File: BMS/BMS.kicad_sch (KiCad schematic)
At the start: 112 parts, among them IC1 L9963E-TR, T1 Transformer_1P_1S, T2 Transformer_1P_1S, U1 QRE1113GR

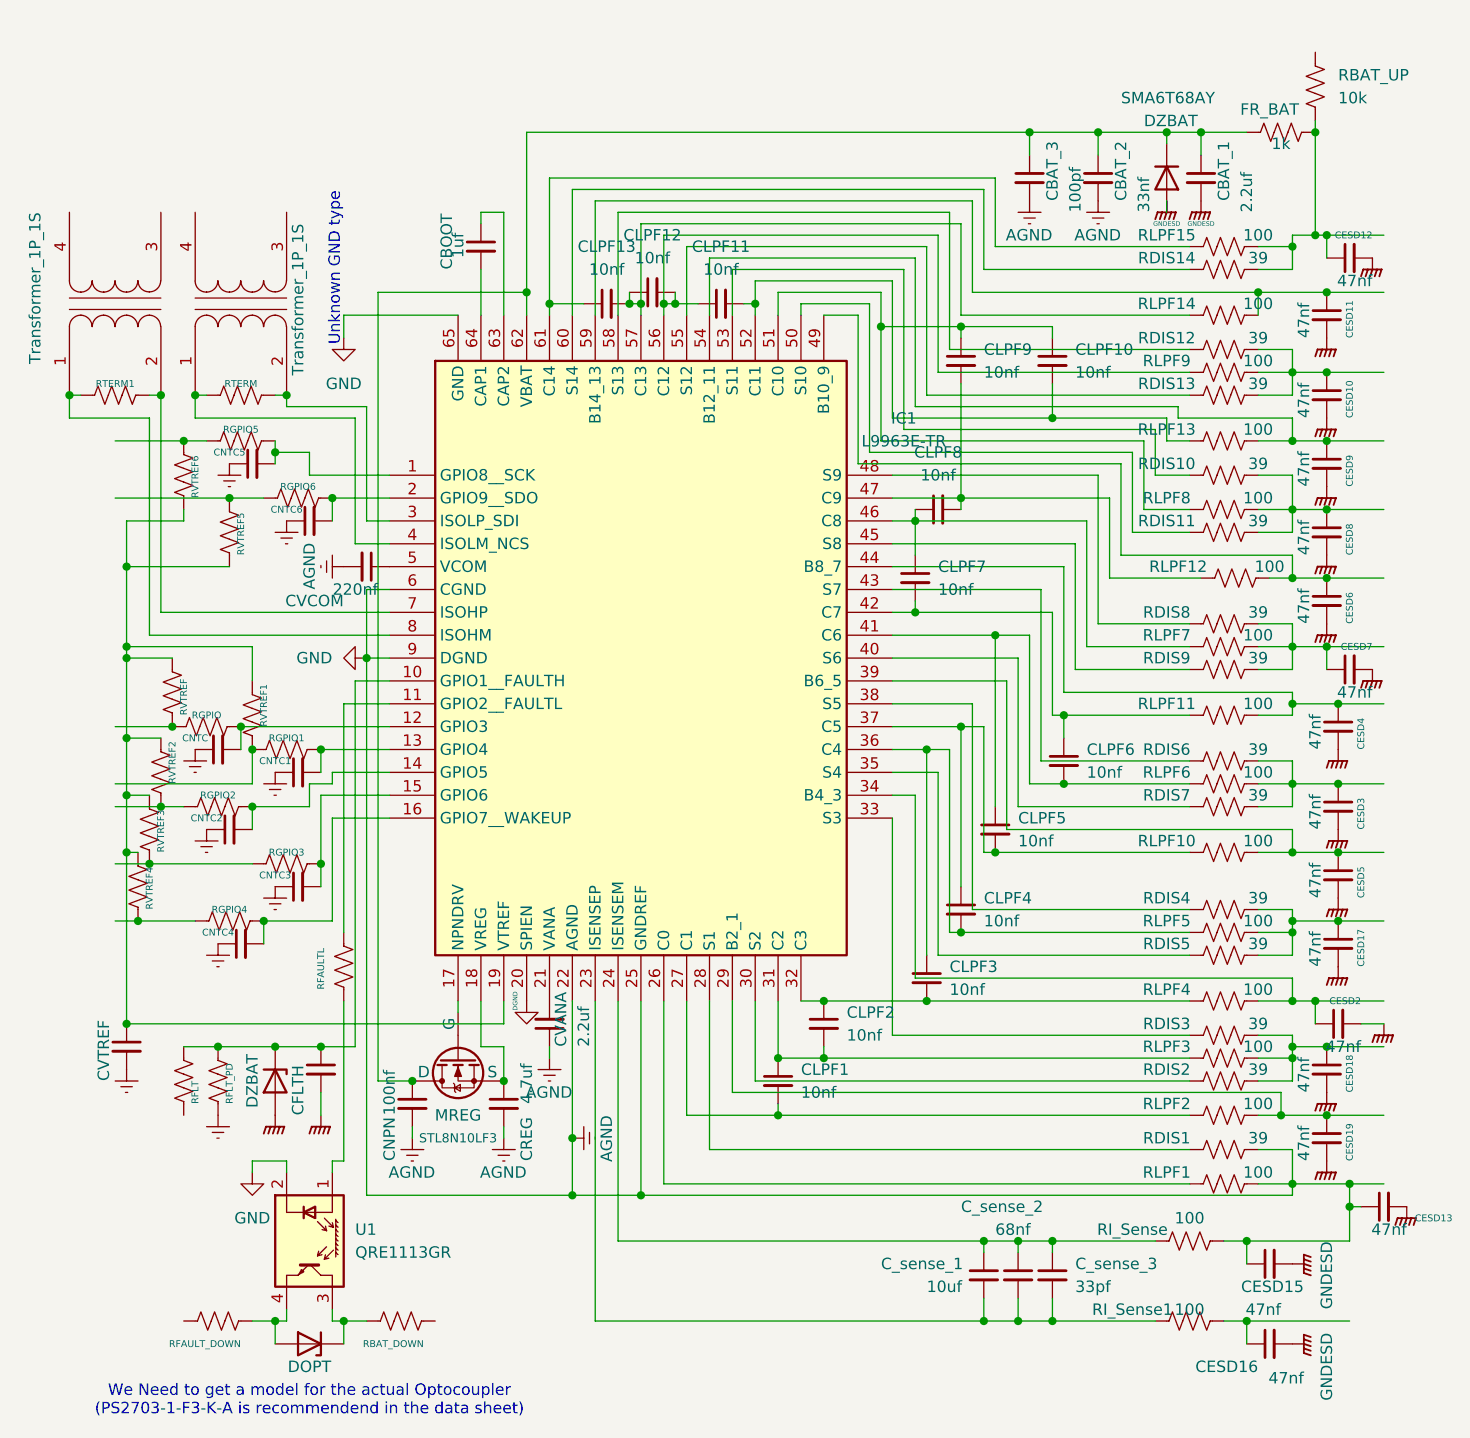
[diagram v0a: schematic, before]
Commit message: Setting up footprint and model library
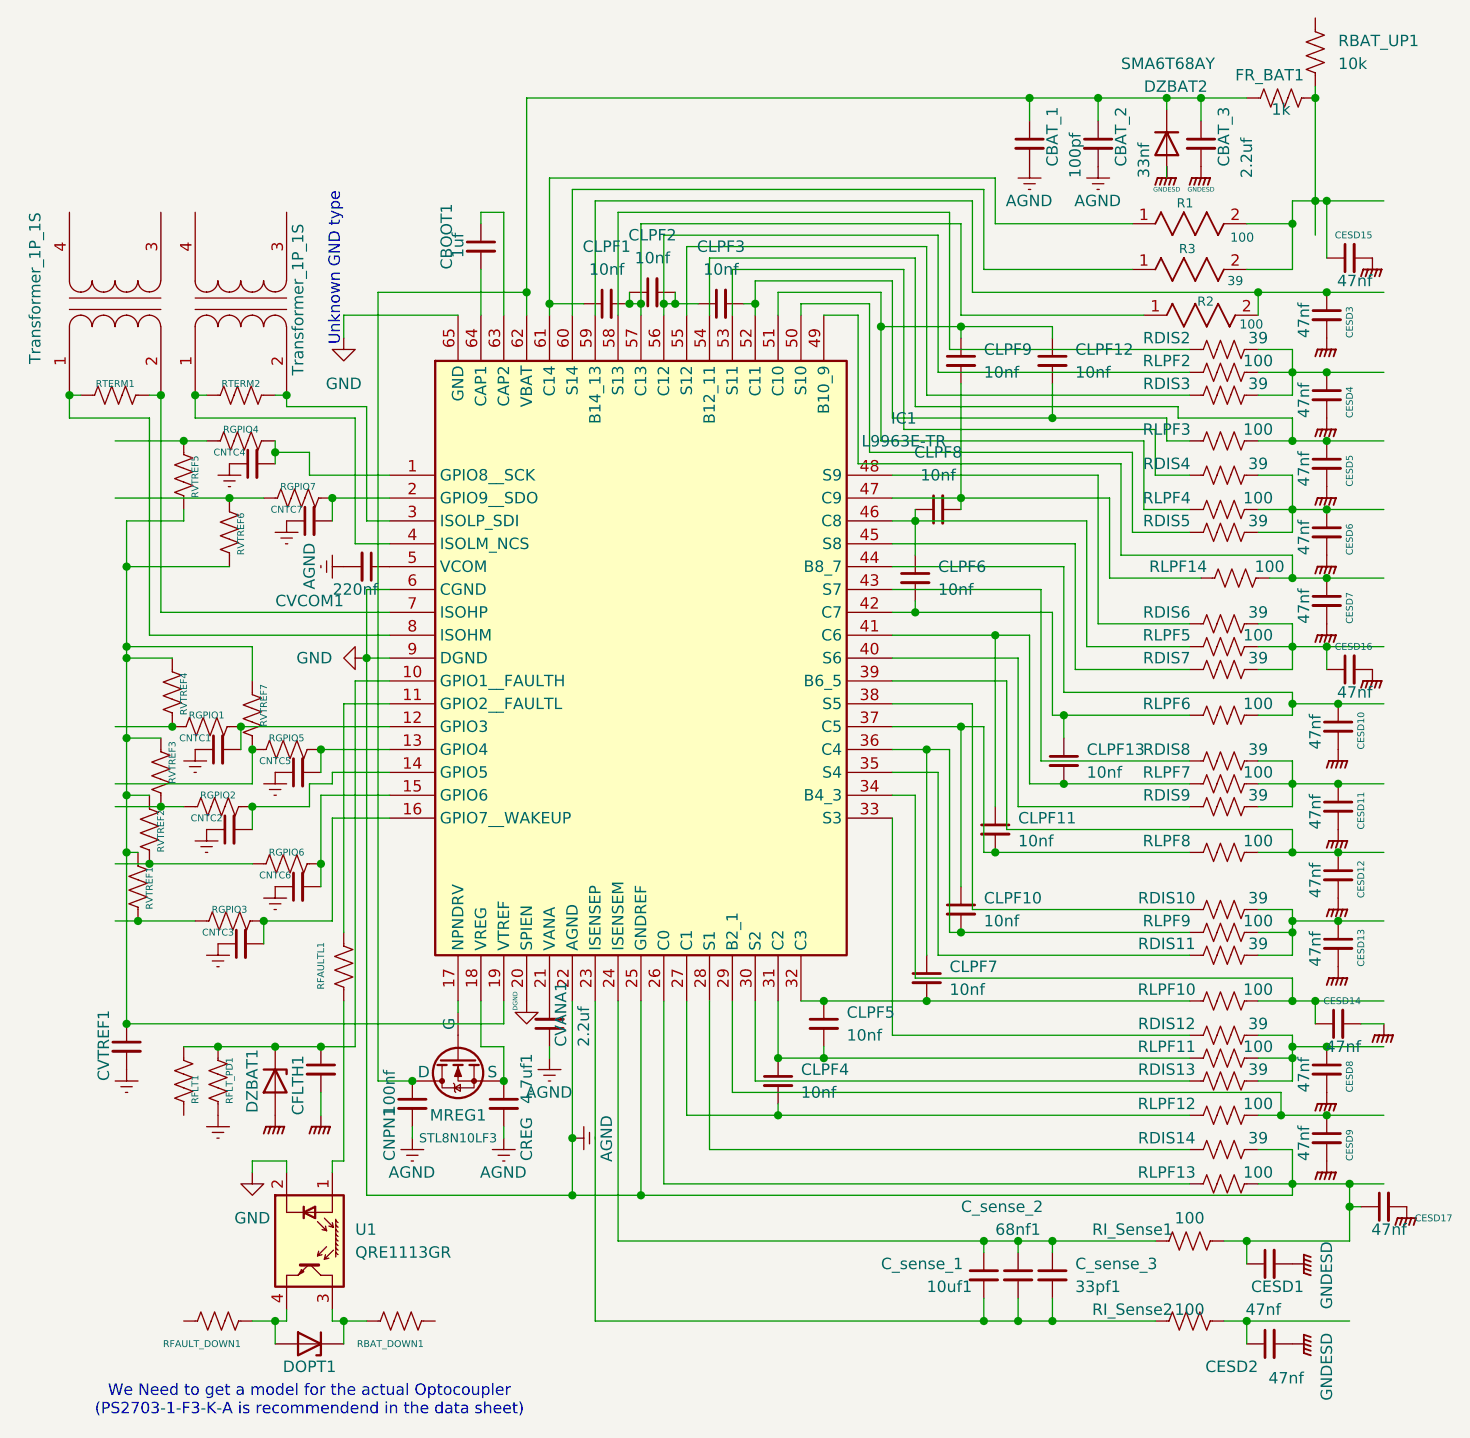
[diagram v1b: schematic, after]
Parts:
- removed RDIS14: 39, symbol Device:R_US
- removed RLPF14, RLPF15: 100, symbol Device:R_US
- added R1, R2: 100, symbol test:RC0603FR-07100RL
- added R3: 39, symbol 39R0603:RC0603FR-0739RL
- IC1: footprint QFP50P1200X1200X120-65N -> R4_standard_footprints:QFP50P1200X1200X120-65N
- renumbered 10uf to 10uf1, 33pf to 33pf1, 4.7uf to 4.7uf1, 68nf to 68nf1, CBAT_3 to CBAT_1, CBAT_1 to CBAT_3, CBOOT to CBOOT1, CESD15 to CESD1, CESD4 to CESD10, CESD3 to CESD11, CESD5 to CESD12, CESD17 to CESD13, CESD2 to CESD14, CESD12 to CESD15, CESD7 to CESD16, CESD13 to CESD17, CESD16 to CESD2, CESD11 to CESD3, CESD10 to CESD4, CESD9 to CESD5, CESD8 to CESD6, CESD6 to CESD7, CESD18 to CESD8, CESD19 to CESD9, CFLTH to CFLTH1, CLPF13 to CLPF1, CLPF4 to CLPF10, CLPF5 to CLPF11, CLPF10 to CLPF12, CLPF6 to CLPF13, CLPF12 to CLPF2, CLPF11 to CLPF3, CLPF1 to CLPF4, CLPF2 to CLPF5, CLPF7 to CLPF6, CLPF3 to CLPF7, CNPN to CNPN1, CNTC to CNTC1, CNTC4 to CNTC3, CNTC5 to CNTC4, CNTC1 to CNTC5, CNTC3 to CNTC6, CNTC6 to CNTC7, CVANA to CVANA1, CVCOM to CVCOM1, CVTREF to CVTREF1, DOPT to DOPT1, DZBAT to DZBAT1, DZBAT to DZBAT2, FR_BAT to FR_BAT1, MREG to MREG1, RBAT_DOWN to RBAT_DOWN1, RBAT_UP to RBAT_UP1, RDIS4 to RDIS10, RDIS5 to RDIS11, RDIS3 to RDIS12, RDIS2 to RDIS13, RDIS1 to RDIS14, RDIS12 to RDIS2, RDIS13 to RDIS3, RDIS10 to RDIS4, RDIS11 to RDIS5, RDIS8 to RDIS6, RDIS9 to RDIS7, RDIS6 to RDIS8, RDIS7 to RDIS9, RFAULTL to RFAULTL1, RFAULT_DOWN to RFAULT_DOWN1, RFLT to RFLT1, RFLT_PD to RFLT_PD1, RGPIO to RGPIO1, RGPIO4 to RGPIO3, RGPIO5 to RGPIO4, RGPIO1 to RGPIO5, RGPIO3 to RGPIO6, RGPIO6 to RGPIO7, RI_Sense to RI_Sense1, RI_Sense1 to RI_Sense2, RLPF4 to RLPF10, RLPF3 to RLPF11, RLPF2 to RLPF12, RLPF1 to RLPF13, RLPF12 to RLPF14, RLPF9 to RLPF2, RLPF13 to RLPF3, RLPF8 to RLPF4, RLPF7 to RLPF5, RLPF11 to RLPF6, RLPF6 to RLPF7, RLPF10 to RLPF8, RLPF5 to RLPF9, RTERM to RTERM2, RVTREF4 to RVTREF1, RVTREF3 to RVTREF2, RVTREF2 to RVTREF3, RVTREF to RVTREF4, RVTREF6 to RVTREF5, RVTREF5 to RVTREF6, RVTREF1 to RVTREF7, T2 to T1, T1 to T2
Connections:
- net at CLPF1.2, CLPF2.1, IC1.57 (C13): now also R2.1
- net at CESD3.1, IC1.59 (B14_13): now also R2.2
- net at CESD15.1, FR_BAT1.2, RBAT_UP1.1: now also R1.2, R3.2
- net at IC1.60 (S14): now also R3.1
- net at CLPF1.1, IC1.61 (C14): now also R1.1
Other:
- moved on the sheet: CBAT_1, CBAT_2, CBAT_3, DZBAT2, FR_BAT1, RBAT_UP1

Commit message: setting up footprints and models (incomplete)
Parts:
- R1, R2: footprint (none) -> R4_standard_footprints:100R-RC0603N_YAG
- R3: footprint (none) -> R4_standard_footprints:39R-RC0603N_YAG
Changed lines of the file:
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@@
 			)
 		)
-		(property "Footprint" ""
+		(property "Footprint" "R4_standard_footprints:39R-RC0603N_YAG"
 			(at 149.86 55.88 0)
 			(effects
@@
 			)
 		)
-		(property "Footprint" ""
+		(property "Footprint" "R4_standard_footprints:100R-RC0603N_YAG"
 			(at 151.13 60.96 0)
 			(effects
@@
 			)
 		)
-		(property "Footprint" ""
+		(property "Footprint" "R4_standard_footprints:100R-RC0603N_YAG"
 			(at 149.86 50.8 0)
 			(effects
